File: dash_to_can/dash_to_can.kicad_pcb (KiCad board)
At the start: 2 copper layers, 63.1 x 77.4 mm, 64 parts, among them J1 AVR-ISP1, J2 Conn_02x10_Top_Bottom, Q1 2N3904, Q10 AO3401A, Q2 2N3904, Q3 2N3904, Q4 AO3401A, Q5 2N3904, Q6 AO3401A, Q7 2N3904, Q8 AO3401A, Q9 2N3904, U1 ATmega328P-A, U2 LM2575-5.0BU, U3 MCP2515-xST, U4 TJA1050T_CM_118, U5 ULN2003A, U6 MCP41010, Y1 20MHz, Y2 16MHz

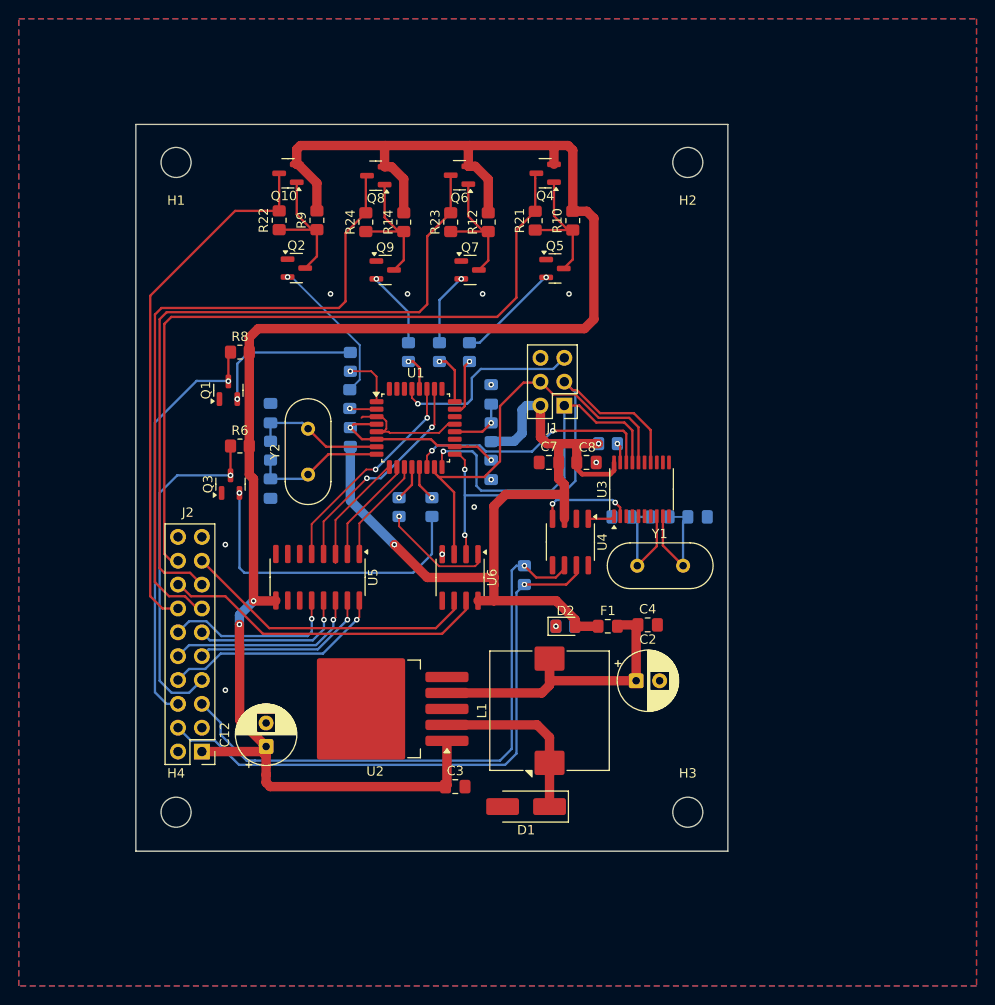
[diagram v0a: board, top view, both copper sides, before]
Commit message: 3rd Draft with Nicholas advice
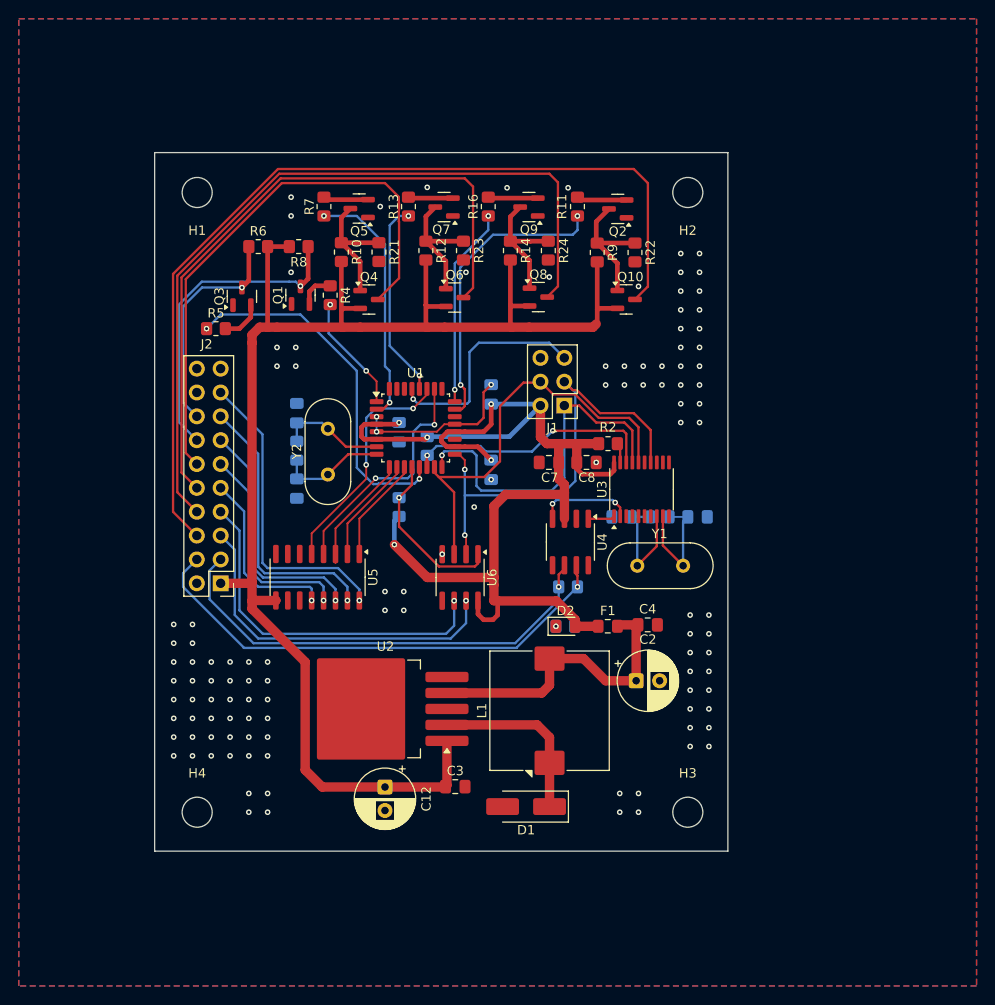
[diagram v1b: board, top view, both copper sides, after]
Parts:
- removed R20: 10k, Resistor_SMD:R_0805_2012Metric_Pad1.20x1.40mm_HandSolder
- added C13: 10uF, Capacitor_SMD:C_0805_2012Metric_Pad1.18x1.45mm_HandSolder, B.Cu at (113.5, 70.5)
- R11, R13, R16, R2, R4, R5, R7: moved to F.Cu
- moved Q10 38.4 mm to (137.7, 56.4), turned to 0 degrees
- moved R22 38.0 mm to (138.6, 51.4), turned to -90 degrees
- moved Q2 34.8 mm to (136.8, 46.8), turned to 180 degrees
- moved R9 30.1 mm to (134.6, 51.4), turned to -90 degrees
- moved R5 29.8 mm to (94.0, 59.5), turned to 0 degrees
- moved R10 24.9 mm to (107.4, 51.3), turned to 90 degrees
- moved Q4 23.1 mm to (110.3, 56.4), turned to 0 degrees
- moved Q5 21.8 mm to (109.3, 46.7), turned to 180 degrees
- moved Q8 21.6 mm to (128.3, 56.1), turned to 0 degrees
- moved R6 21.3 mm to (98.5, 50.8)
- moved R7 20.7 mm to (105.5, 46.5)
- moved Q3 20.0 mm to (96.8, 56.1)
- moved R24 19.7 mm to (129.4, 51.2), turned to -90 degrees
- moved R11 19.3 mm to (132.5, 46.5)
- moved J2 18.0 mm to (94.5, 86.6)
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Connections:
- C1 pad 1: Net-(U1-AVCC) -> +5V
- C11 pad 2: Net-(U1-AREF) -> +5V
- J2 pad 10: FI IND -> TURN R
- J2 pad 12: IMMOBI IND -> TURN L
- J2 pad 13: TURN R -> FI IND
- J2 pad 14: TURN L -> SP
- J2 pad 15: HI BEAM -> Oil
- J2 pad 16: TEMP -> TACHO
- J2 pad 17: FUEL -> Neutral
- J2 pad 18: ILLUM -> unconnected-(J2-Pin_18-Pad18)
- J2 pad 2: unconnected-(J2-Pin_2-Pad2) -> GND
- J2 pad 3: GND -> CANL
- J2 pad 5: CANL -> TEMP
- J2 pad 6: SP -> ILLUM
- J2 pad 7: TACHO -> FUEL
- J2 pad 8: Neutral -> HI BEAM
- J2 pad 9: Oil -> IMMOBI IND
- Q1 pad 2: SP_OUT -> Net-(Q1-B)
- Q10 pad 3: TURN L -> ILLUM
- Q2 pad 2: L DRIVER -> Net-(Q2-B)
- Q3 pad 2: TACHO DRIVER -> Net-(Q3-B)
- Q4 pad 3: ILLUM -> TURN L
- Q5 pad 2: ILLUM DRIVER -> Net-(Q5-B)
- Q6 pad 3: HI BEAM -> TURN R
- Q7 pad 2: HI BEAM DRIVER -> Net-(Q7-B)
- Q8 pad 3: TURN R -> HI BEAM
- Q9 pad 2: R DRIVER -> Net-(Q9-B)
- R11 pad 1: Net-(U1-PC0) -> ILLUM DRIVER
- R11 pad 2: ILLUM DRIVER -> Net-(Q2-B)
- R13 pad 1: Net-(U1-PC5) -> R DRIVER
- R13 pad 2: R DRIVER -> Net-(Q7-B)
- R16 pad 1: Net-(U1-PC1) -> Net-(Q9-B)
- R18 pad 1: Net-(U1-AREF) -> CS_CAN
- R19 pad 1: Net-(U1-PB0) -> CS_MCP41
- R19 pad 2: CS -> +5V
- R21 pad 2: ILLUM -> GND
- R22 pad 2: TURN L -> GND
- R23 pad 2: HI BEAM -> GND
- R24 pad 2: TURN R -> GND
- R4 pad 1: Net-(U1-PD3) -> SP_OUT
- R4 pad 2: SP_OUT -> Net-(Q1-B)
- R5 pad 1: Net-(U1-PB1) -> TACHO DRIVER
- R5 pad 2: TACHO DRIVER -> Net-(Q3-B)
- R7 pad 1: Net-(U1-PD4) -> L DRIVER
- R7 pad 2: L DRIVER -> Net-(Q5-B)
- U1 pad 1: Net-(U1-PD3) -> SP_OUT
- U1 pad 12: Net-(U1-PB0) -> CS_MCP41
- U1 pad 13: Net-(U1-PB1) -> TACHO DRIVER
- U1 pad 14: CS2 -> CS_CAN
- U1 pad 18: Net-(U1-AVCC) -> +5V
- U1 pad 2: Net-(U1-PD4) -> L DRIVER
- U1 pad 20: Net-(U1-AREF) -> +5V
- U1 pad 23: Net-(U1-PC0) -> ILLUM DRIVER
- U1 pad 24: Net-(U1-PC1) -> HI BEAM DRIVER
- U1 pad 28: Net-(U1-PC5) -> R DRIVER
- U1 pad 4: Net-(U1-AVCC) -> +5V
- U1 pad 6: Net-(U1-AVCC) -> +5V
- U3 pad 18: CS2 -> CS_CAN
- U6 pad 1: CS -> CS_MCP41
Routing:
- net +12V: track 196.7 -> 160.1 mm, vias 2 -> 0
- net +5V: track 91.8 -> 123.5 mm, vias 2 -> 5
- net CS2: track 27.3 -> 0.00 mm, vias 2 -> 0
- net CS_CAN: track 0.00 -> 27.2 mm, vias 0 -> 2
- net ILLUM DRIVER: track 11.0 -> 31.8 mm, vias 1 -> 2
- net Net-(U1-AVCC): track 19.4 -> 0.00 mm, vias 2 -> 0
- net ILLUM: track 79.0 -> 97.7 mm
- net CS_MCP41: track 0.00 -> 18.2 mm, vias 0 -> 1
- net HI BEAM DRIVER: track 7.66 -> 21.3 mm, vias 1 -> 2
- net CANL: track 63.5 -> 50.3 mm
- net TACHO: track 37.0 -> 24.1 mm
- net R DRIVER: track 8.20 -> 21.1 mm, vias 1 -> 2
- net CS: track 12.3 -> 0.00 mm, vias 1 -> 0
- net SP: track 44.9 -> 34.0 mm
- net L DRIVER: track 15.9 -> 26.5 mm, vias 1 -> 2
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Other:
- board size 63.1 x 77.4 mm -> 61.1 x 74.4 mm
